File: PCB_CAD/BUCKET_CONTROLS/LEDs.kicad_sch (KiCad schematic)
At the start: 120 parts, among them J1 Pow, J10 Data, J101 Pow, J102 Data, J103 Pow, J104 Data, J105 Pow, J106 Data, J107 Pow, J108 Data, J109 Pow, J11 Pow, J110 Data, J111 Pow, J112 Data, J113 Pow, J114 Data, J115 Pow, J116 Data, J117 Pow, J118 Data, J119 Pow, J12 Data, J120 Data, J13 Pow, J14 Data, J15 Pow, J16 Data, J17 Pow, J18 Data, J19 Pow, J2 Data, J20 Data, J201 Pow, J202 Data, J203 Pow, J204 Data, J205 Pow, J206 Data, J207 Pow, J208 Data, J209 Pow, J210 Data, J211 Pow, J212 Data, J213 Pow, J214 Data, J215 Pow, J216 Data, J217 Pow, J218 Data, J219 Pow, J220 Data, J3 Pow, J301 Pow, J302 Data, J303 Pow, J304 Data, J305 Pow, J306 Data, J307 Pow, J308 Data, J309 Pow, J310 Data, J311 Pow, J312 Data, J313 Pow, J314 Data, J315 Pow, J316 Data, J317 Pow, J318 Data, J319 Pow, J320 Data, J4 Data, J5 Pow, J6 Data, J7 Pow, J8 Data, J9 Pow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

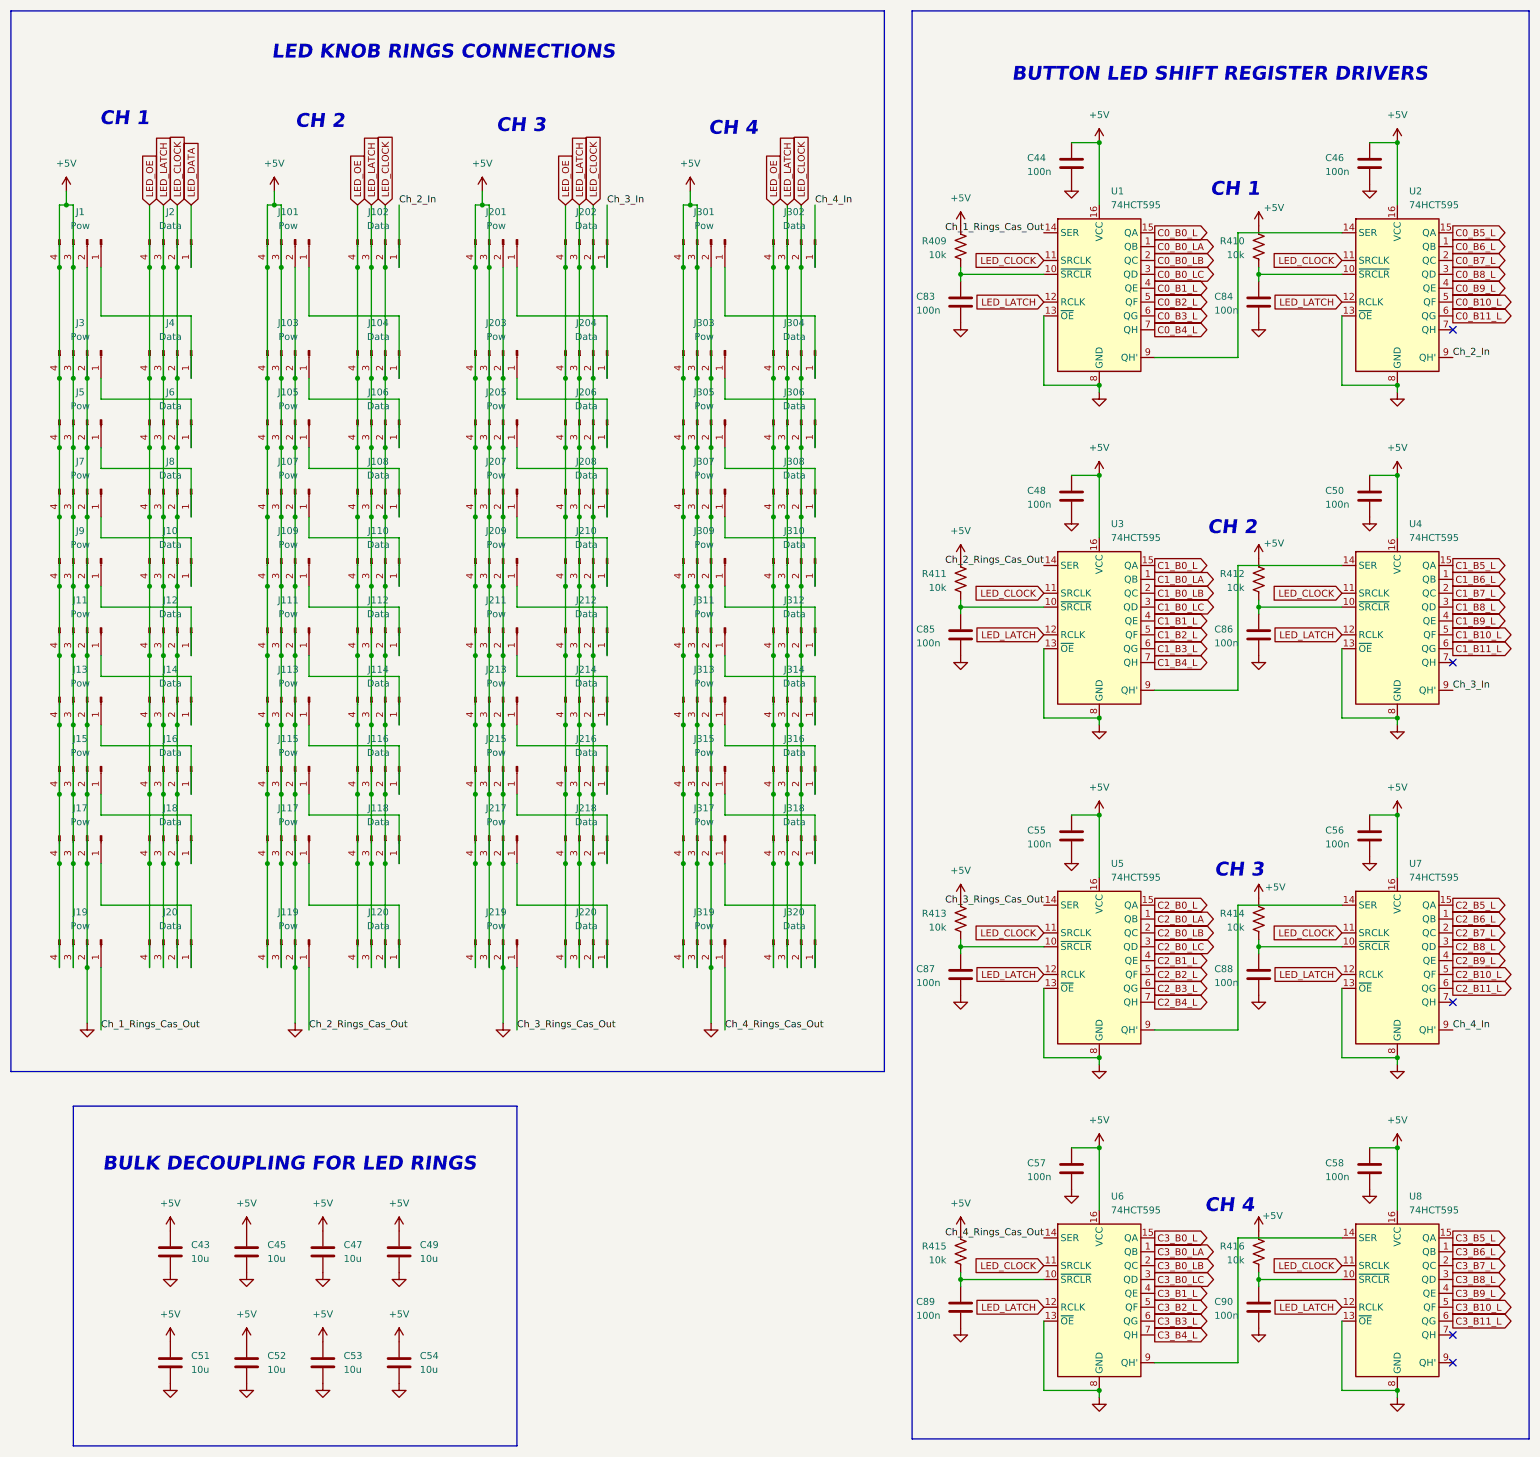
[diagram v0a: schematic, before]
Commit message: save pcb progress lol
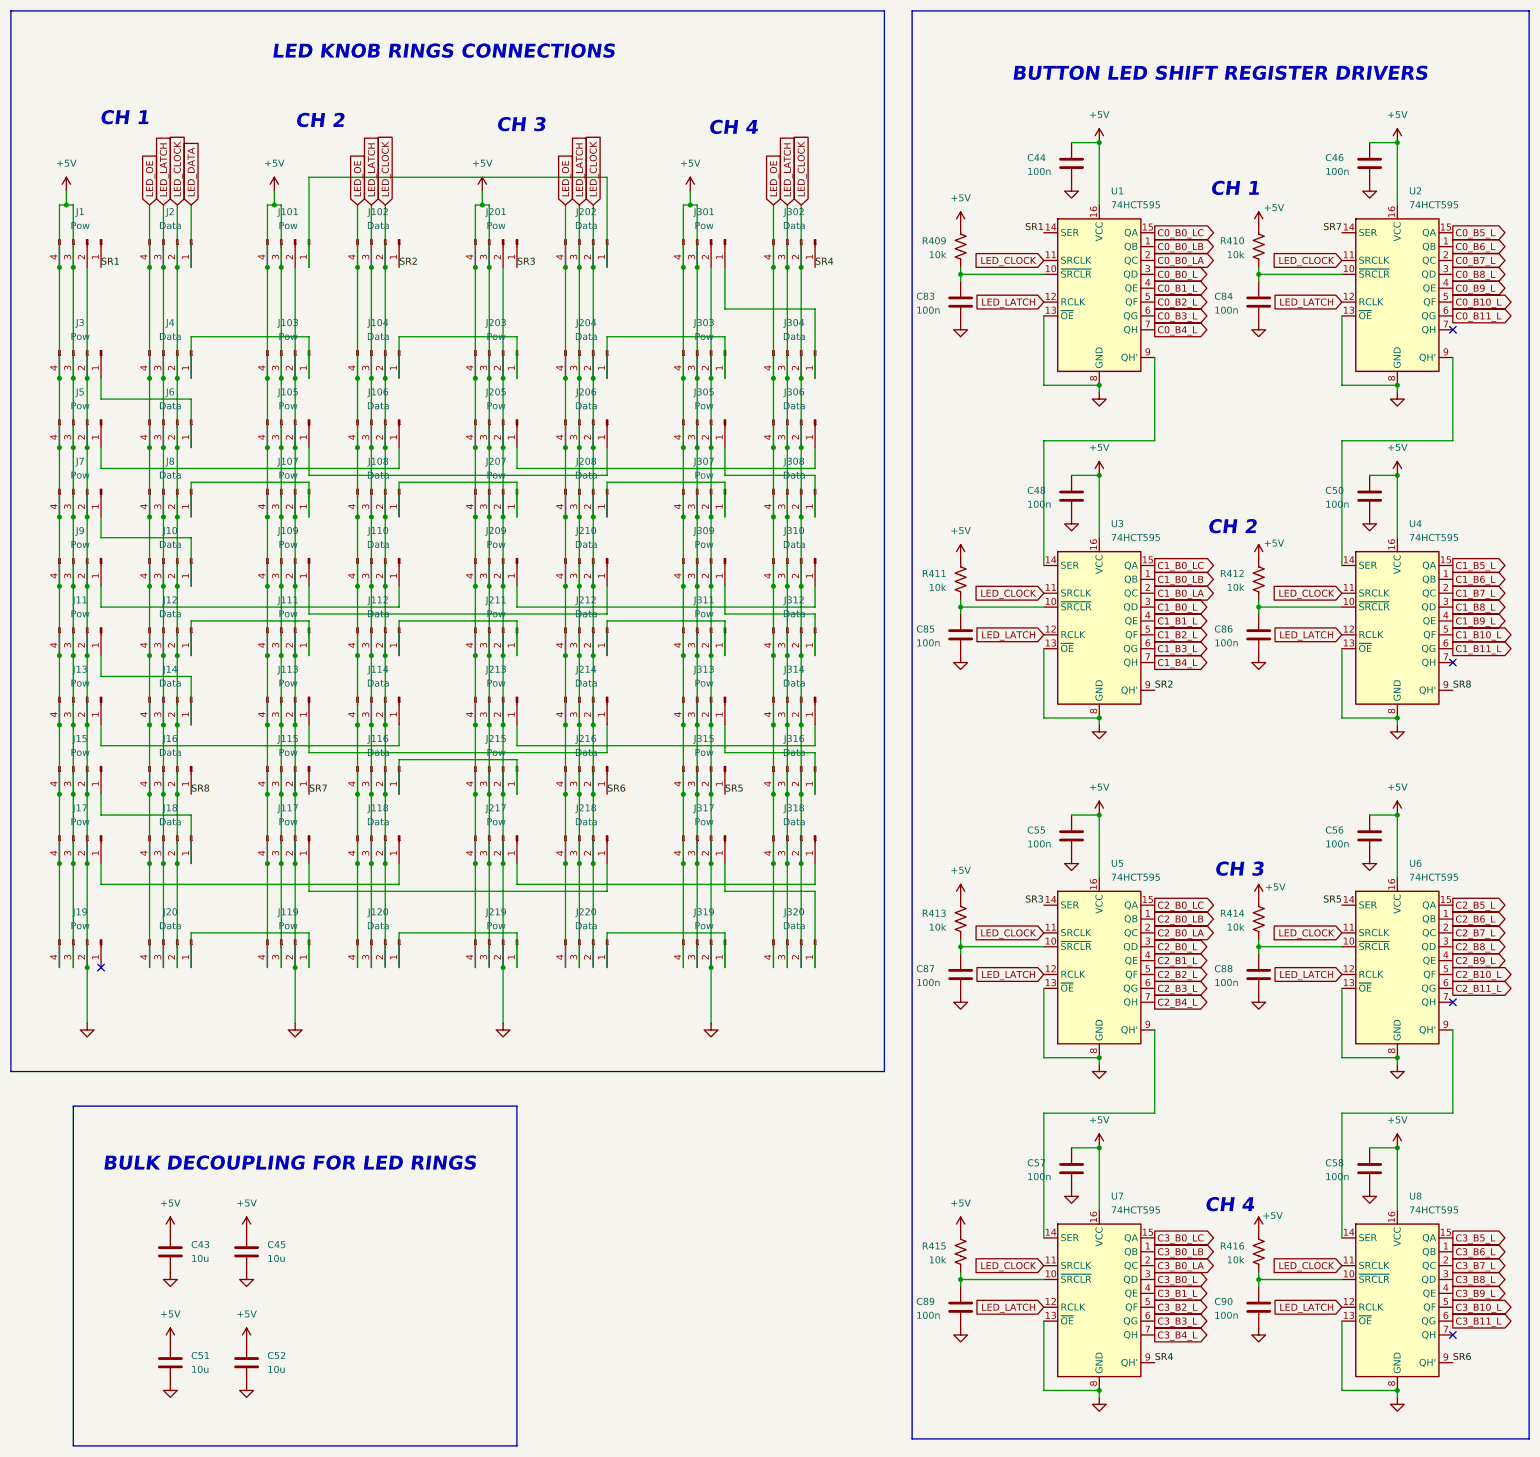
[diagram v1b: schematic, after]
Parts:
- removed C47, C49, C53, C54: 10u, Capacitor_SMD:C_0603_1608Metric, symbol Device:C
- renumbered U7 to U6, U6 to U7
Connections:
- net C0_B0_L: now also U1.3 (QD); no longer U1.15 (QA)
- net C0_B0_LA: now also U1.2 (QC); no longer U1.1 (QB)
- net C0_B0_LB: now also U1.1 (QB); no longer U1.2 (QC)
- net C0_B0_LC: now also U1.15 (QA); no longer U1.3 (QD)
- net C1_B0_L: now also U3.3 (QD); no longer U3.15 (QA)
- net C1_B0_LA: now also U3.2 (QC); no longer U3.1 (QB)
- net C1_B0_LB: now also U3.1 (QB); no longer U3.2 (QC)
- net C1_B0_LC: now also U3.15 (QA); no longer U3.3 (QD)
- net C2_B0_L: now also U5.3 (QD); no longer U5.15 (QA)
- net C2_B0_LA: now also U5.2 (QC); no longer U5.1 (QB)
- net C2_B0_LB: now also U5.1 (QB); no longer U5.2 (QC)
- net C2_B0_LC: now also U5.15 (QA); no longer U5.3 (QD)
- net C3_B0_L: now also U7.3 (QD); no longer U7.15 (QA)
- net C3_B0_LA: now also U7.2 (QC); no longer U7.1 (QB)
- net C3_B0_LB: now also U7.1 (QB); no longer U7.2 (QC)
- net C3_B0_LC: now also U7.15 (QA); no longer U7.3 (QD)
- net at J318.1 (Pin_1): now also J217.1 (Pin_1); no longer J315.1 (Pin_1)
- net at J314.1 (Pin_1): now also J213.1 (Pin_1); no longer J311.1 (Pin_1)
- net at J17.1 (Pin_1): now also J118.1 (Pin_1); no longer J20.1 (Pin_1)
- net at J215.1 (Pin_1): now also J116.1 (Pin_1); no longer J218.1 (Pin_1)
- net at J103.1 (Pin_1): now also J4.1 (Pin_1); no longer J106.1 (Pin_1)
- net SR6: now reaches J216.1 (Pin_1)
- net SR6: now also U8.9 (QH'); no longer J213.1 (Pin_1)
- net at J113.1 (Pin_1): now also J214.1 (Pin_1); no longer J116.1 (Pin_1)
- net at J220.1 (Pin_1): now also J319.1 (Pin_1); no longer J217.1 (Pin_1)
- net at U5.9 (QH'): now also U7.14 (SER); no longer U6.14 (SER)
- net at J114.1 (Pin_1): now also J13.1 (Pin_1); no longer J111.1 (Pin_1)
- net at J117.1 (Pin_1): now also J218.1 (Pin_1); no longer J120.1 (Pin_1)
- net at U1.9 (QH'): now also U3.14 (SER); no longer U2.14 (SER)
- net at J310.1 (Pin_1): now also J209.1 (Pin_1); no longer J307.1 (Pin_1)
- net SR8: now reaches J16.1 (Pin_1)
- net SR8: now also U4.9 (QH'); no longer J13.1 (Pin_1)
- net at U8.14 (SER): now also U6.9 (QH'); no longer U7.9 (QH')
- net SR1: now reaches J1.1 (Pin_1)
- net SR1: now also U1.14 (SER); no longer J4.1 (Pin_1)
- net at J204.1 (Pin_1): now also J303.1 (Pin_1); no longer J201.1 (Pin_1)
- net at U4.14 (SER): now also U2.9 (QH'); no longer U3.9 (QH')
- net at J211.1 (Pin_1): now also J112.1 (Pin_1); no longer J214.1 (Pin_1)
- net at J9.1 (Pin_1): now also J110.1 (Pin_1); no longer J12.1 (Pin_1)
- net SR7: now reaches J115.1 (Pin_1)
- net SR7: now also U2.14 (SER); no longer J118.1 (Pin_1)
- net at J203.1 (Pin_1): now also J104.1 (Pin_1); no longer J206.1 (Pin_1)
- net at J208.1 (Pin_1): now also J307.1 (Pin_1); no longer J205.1 (Pin_1)
- net at J212.1 (Pin_1): now also J311.1 (Pin_1); no longer J209.1 (Pin_1)
- net at J101.1 (Pin_1): now also J202.1 (Pin_1); no longer J104.1 (Pin_1)
- net at J306.1 (Pin_1): now also J205.1 (Pin_1); no longer J303.1 (Pin_1)
- net at J207.1 (Pin_1): now also J108.1 (Pin_1); no longer J210.1 (Pin_1)
- net at J107.1 (Pin_1): now also J8.1 (Pin_1); no longer J110.1 (Pin_1)
- net at J105.1 (Pin_1): now also J206.1 (Pin_1); no longer J108.1 (Pin_1)
- net at J5.1 (Pin_1): now also J106.1 (Pin_1); no longer J8.1 (Pin_1)
- net at J109.1 (Pin_1): now also J210.1 (Pin_1); no longer J112.1 (Pin_1)
- net Ch_1_Rings_Cas_Out: no longer names the net of J19.1 (Pin_1)
- net Ch_1_Rings_Cas_Out: no longer U1.14 (SER)
- net Ch_2_In renamed SR2
- net SR2: now also U3.9 (QH'); no longer U2.9 (QH')
- net Ch_2_Rings_Cas_Out: no longer names the net of J119.1 (Pin_1)
- net Ch_2_Rings_Cas_Out: now also J20.1 (Pin_1); no longer U3.14 (SER)
- removed net Ch_3_In: J202.1 (Pin_1), U4.9 (QH')
- net Ch_3_Rings_Cas_Out: no longer names the net of J219.1 (Pin_1)
- net Ch_3_Rings_Cas_Out: now also J120.1 (Pin_1); no longer U5.14 (SER)
- net Ch_4_In renamed SR4
- net SR4: now also U7.9 (QH'); no longer U6.9 (QH')
- removed net Ch_4_Rings_Cas_Out: J319.1 (Pin_1), U7.14 (SER)
- new net: J111.1 (Pin_1), J12.1 (Pin_1)
- new net SR3: J201.1 (Pin_1), U5.14 (SER)
- new net SR5: J315.1 (Pin_1), U6.14 (SER)

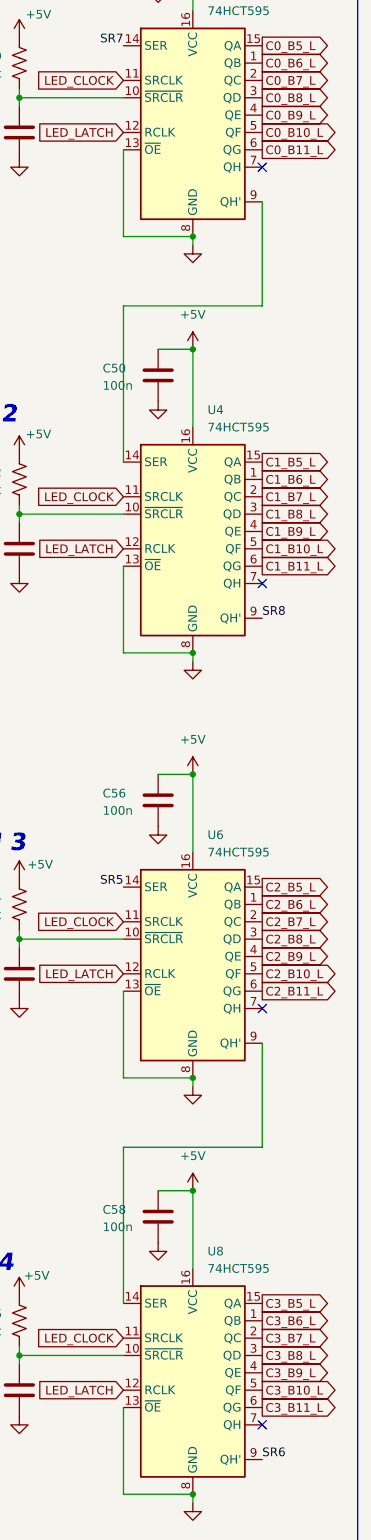
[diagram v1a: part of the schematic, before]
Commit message: pcb routing all day
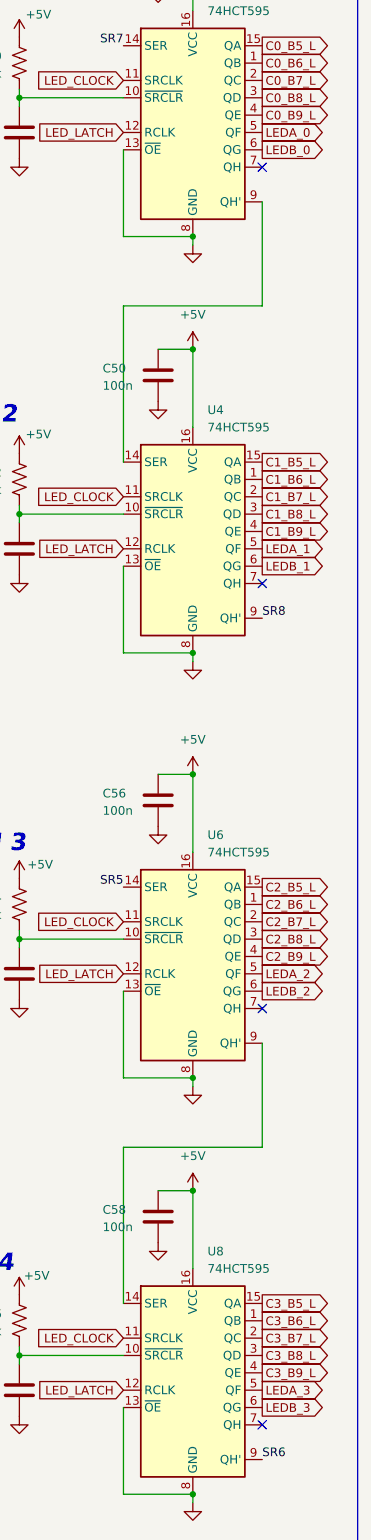
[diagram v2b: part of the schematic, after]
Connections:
- net C0_B10_L renamed LEDA_0
- net C0_B11_L renamed LEDB_0
- net C1_B10_L renamed LEDA_1
- net C1_B11_L renamed LEDB_1
- net C2_B10_L renamed LEDA_2
- net C2_B11_L renamed LEDB_2
- net C3_B10_L renamed LEDA_3
- net C3_B11_L renamed LEDB_3
